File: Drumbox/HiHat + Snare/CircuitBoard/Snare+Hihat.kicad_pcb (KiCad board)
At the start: 2 copper layers, 127.5 x 133 mm, 85 parts, among them J1 Snare IN, J10 Conn_01x03_Female, J11 Conn_01x03_Male, J2 Power Input, J3 HiHat IN, J4 Snare OUT, J5 Conn_01x08_Male, J6 Conn_01x08_Female, J7 Conn_01x08_Male, J8 Conn_01x08_Female, J9 HiHat OUT, Q1 BC546, Q2 BC546, Q3 BC546, Q4 2N3904, Q5 BC546, Q6 BC546, Q7 BC546, Q8 2N3904, U1 TL072

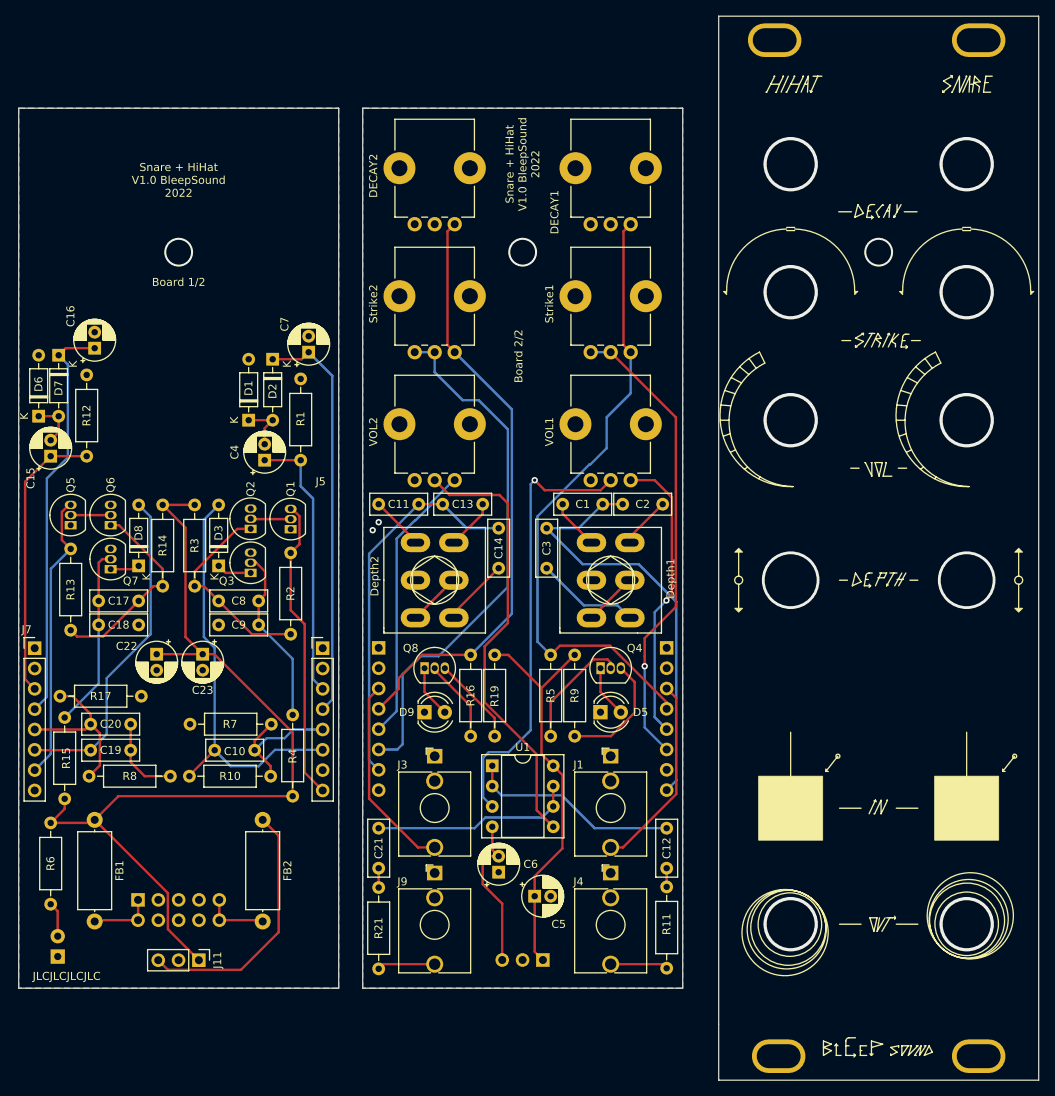
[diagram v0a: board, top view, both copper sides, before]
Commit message: update gerber for all boards on hihat + snare
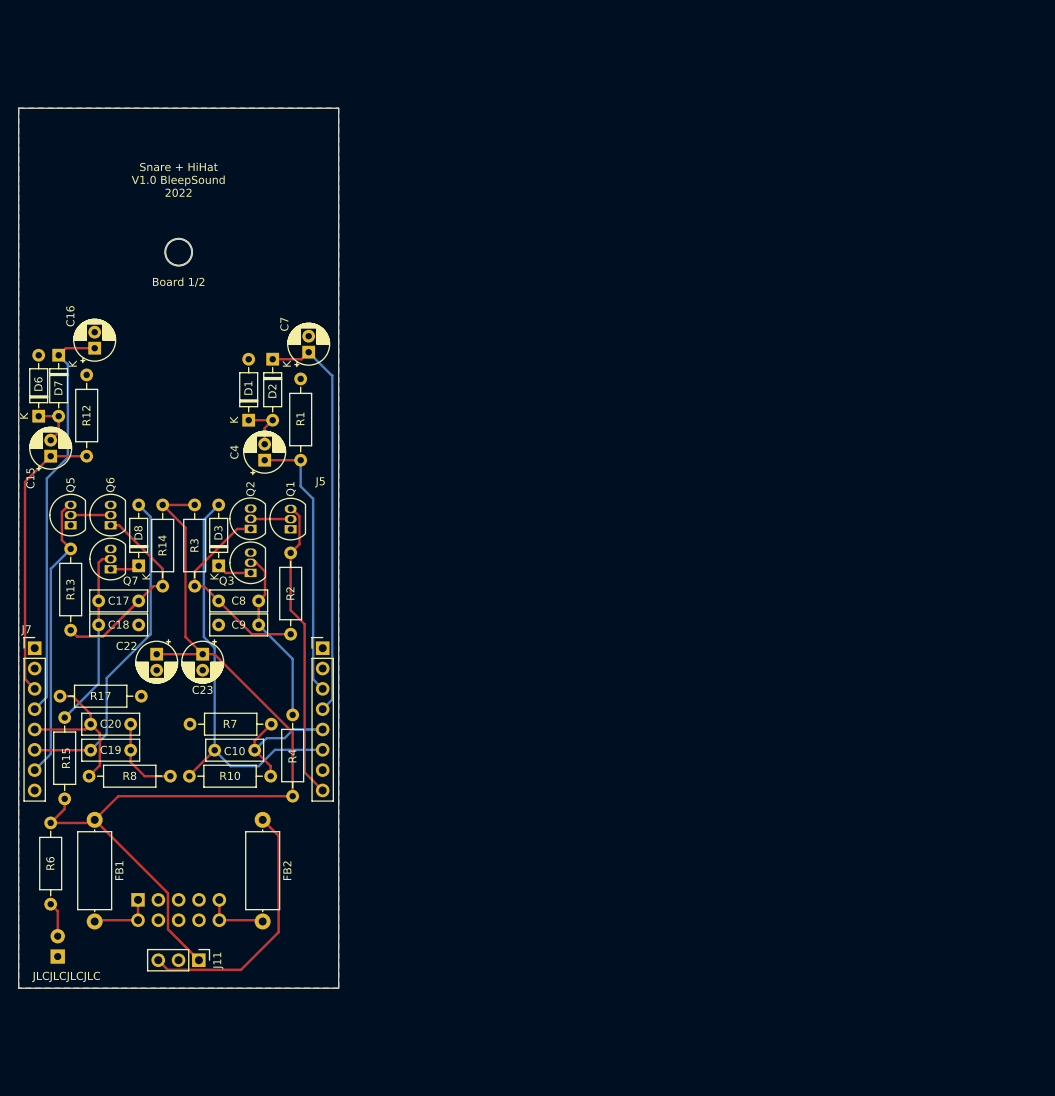
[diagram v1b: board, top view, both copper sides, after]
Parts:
- removed C1, C11, C12, C21: 10µF, Capacitor_THT:C_Disc_D7.0mm_W2.5mm_P5.00mm
- removed C13, C2: 1µF, Capacitor_THT:C_Disc_D7.0mm_W2.5mm_P5.00mm
- removed C14, C3: 0.1µF, Capacitor_THT:C_Disc_D7.0mm_W2.5mm_P5.00mm
- removed C5, C6: 10µ, Capacitor_THT:CP_Radial_D5.0mm_P2.00mm
- removed D5: Trig Snare, LED_THT:LED_D4.0mm
- removed D9: Trig_HiHat, LED_THT:LED_D4.0mm
- removed DECAY1, DECAY2, Strike1, Strike2: 100k, Potentiometer_THT:Potentiometer_Bourns_PTV09A-1_Single_Vertical
- removed Depth1, Depth2: SW_Push_DPDT, Synth:SW_DPDT_Toggle
- removed J1: Snare IN, Connector_Audio:Jack_3.5mm_QingPu_WQP-PJ398SM_Vertical_CircularHoles
- removed J10: Conn_01x03_Female, Connector_PinSocket_2.54mm:PinSocket_1x03_P2.54mm_Vertical
- removed J3: HiHat IN, Connector_Audio:Jack_3.5mm_QingPu_WQP-PJ398SM_Vertical_CircularHoles
- removed J4: Snare OUT, Connector_Audio:Jack_3.5mm_QingPu_WQP-PJ398SM_Vertical_CircularHoles
- removed J6, J8: Conn_01x08_Female, Connector_PinSocket_2.54mm:PinSocket_1x08_P2.54mm_Vertical
- removed J9: HiHat OUT, Connector_Audio:Jack_3.5mm_QingPu_WQP-PJ398SM_Vertical_CircularHoles
- removed Q4, Q8: 2N3904, Package_TO_SOT_THT:TO-92_Inline
- removed R11, R19, R21, R9: 1k, Resistor_THT:R_Axial_DIN0207_L6.3mm_D2.5mm_P10.16mm_Horizontal
- removed R16, R5: 100k, Resistor_THT:R_Axial_DIN0207_L6.3mm_D2.5mm_P10.16mm_Horizontal
- removed REF** (x4): Doepfer Mounting hole, Synth:Doepfer Mounting hole
- removed U1: TL072, Package_DIP:DIP-8_W7.62mm_Socket
- removed VOL1, VOL2: 10k, Potentiometer_THT:Potentiometer_Bourns_PTV09A-1_Single_Vertical
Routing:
- net /SnH: track 130.1 -> 51.2 mm
- net /HiH: track 126.0 -> 51.3 mm
- net /Ho: track 107.9 -> 41.4 mm
- net /So: track 110.0 -> 51.7 mm, vias 1 -> 0
- net Net-(VOL1-Pad2): track 55.9 -> 0.00 mm, vias 1 -> 0
- net Net-(VOL2-Pad2): track 55.5 -> 0.00 mm
- net /DeH: track 92.7 -> 37.9 mm
- net +12V: track 162.4 -> 112.0 mm
- net /HiDH: track 83.6 -> 36.1 mm
- net /SnO: track 54.3 -> 17.8 mm, vias 1 -> 0
- net /HiO: track 56.0 -> 20.8 mm
- net Net-(U1-Pad2): track 26.5 -> 0.00 mm
- net Net-(C21-Pad1): track 25.5 -> 0.00 mm
- net /HiI: track 60.4 -> 35.4 mm
- net /SnI: track 58.9 -> 34.2 mm
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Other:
- board size 127.5 x 133 mm -> 40 x 110 mm
- board text removed: "Board 2/2"
